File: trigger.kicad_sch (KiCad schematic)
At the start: 6 parts, among them K7 Relay_SPDT, U2 LTC6754xSC6

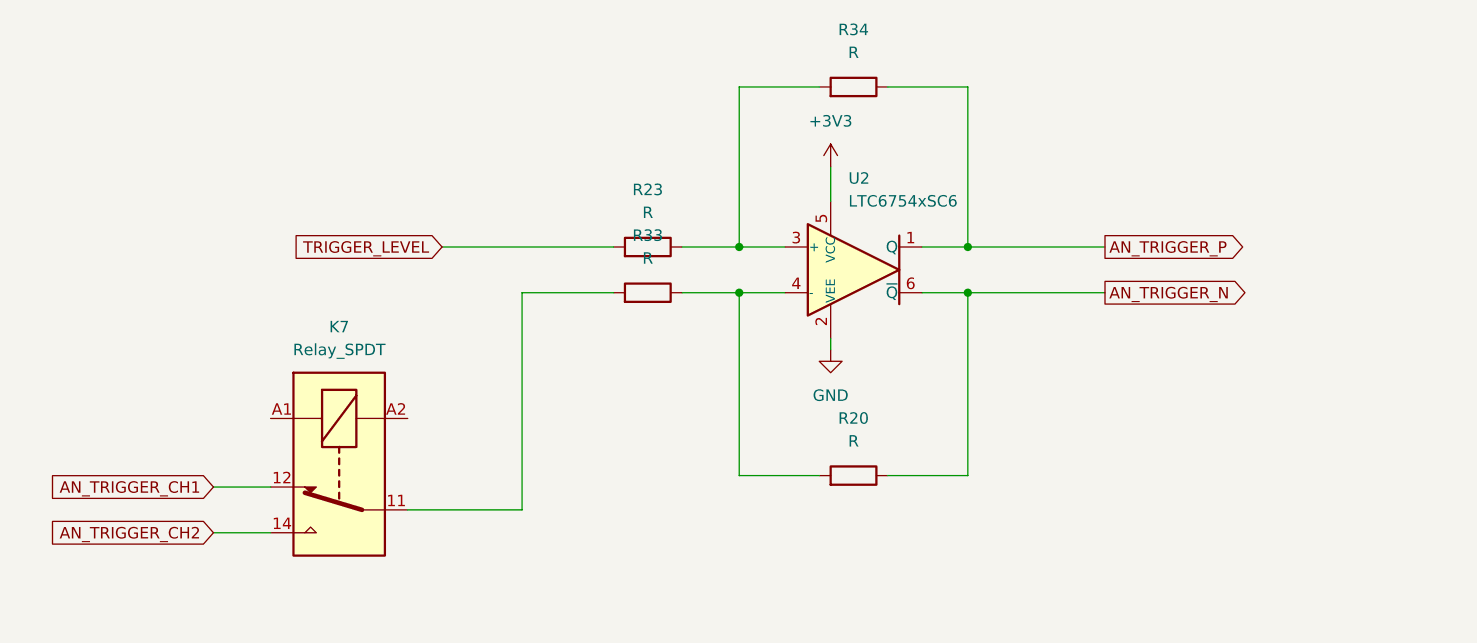
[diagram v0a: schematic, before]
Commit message: Add things to MCU on the board
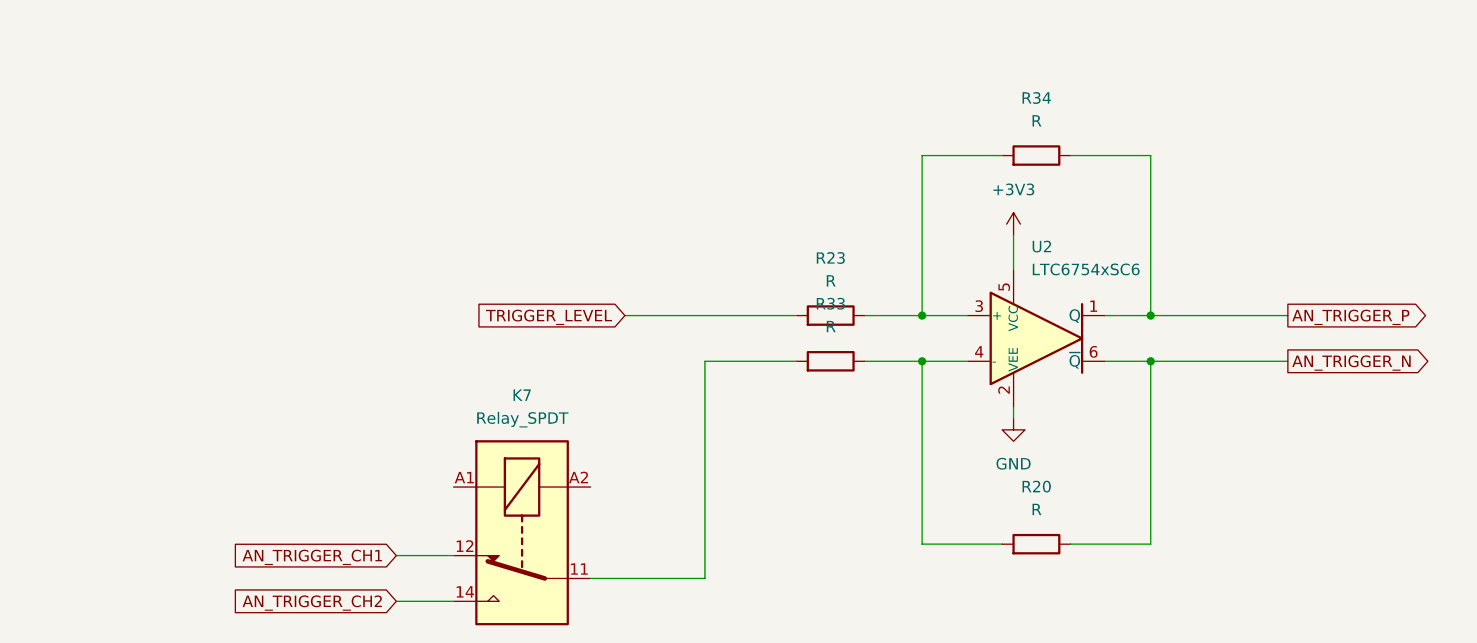
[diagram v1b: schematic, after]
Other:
- moved on the sheet: K7, R20, R23, R33, R34, U2
